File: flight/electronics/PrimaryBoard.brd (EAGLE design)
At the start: 90 x 90 mm, 14 parts

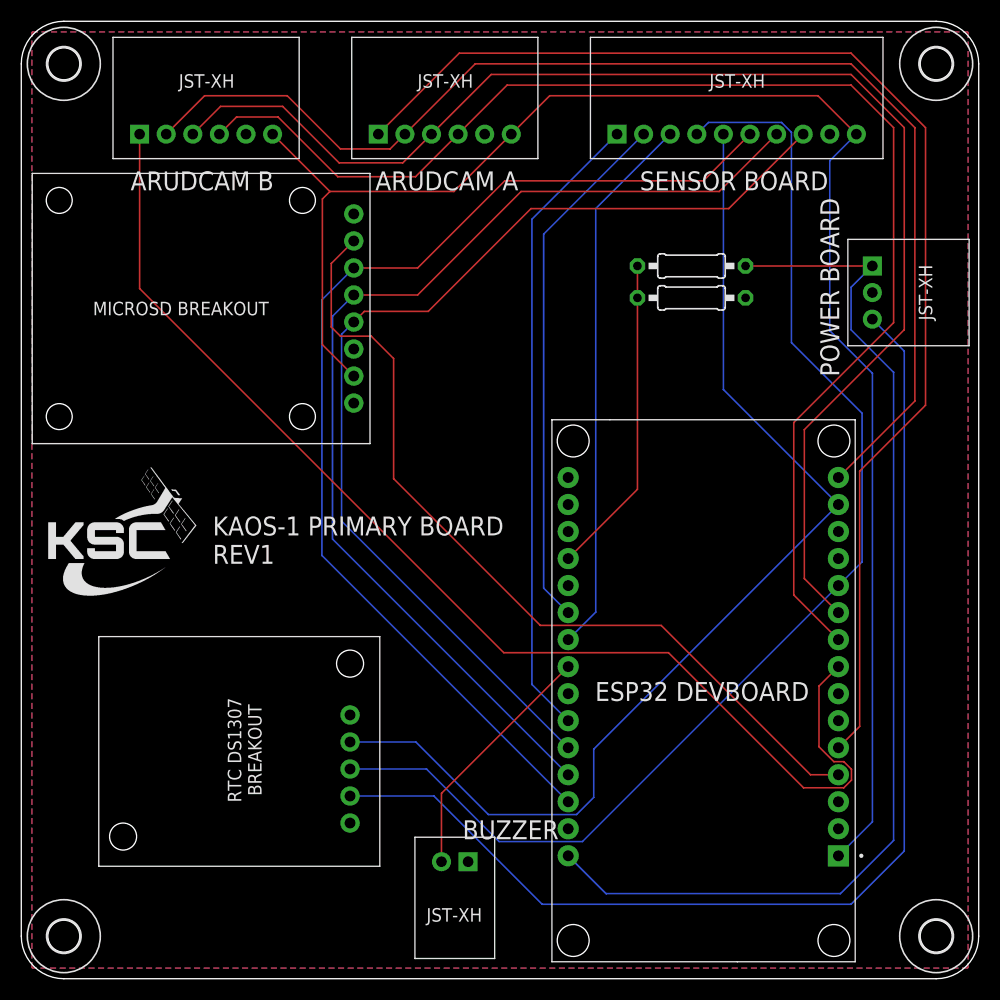
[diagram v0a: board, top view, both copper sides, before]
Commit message: primary board redesign
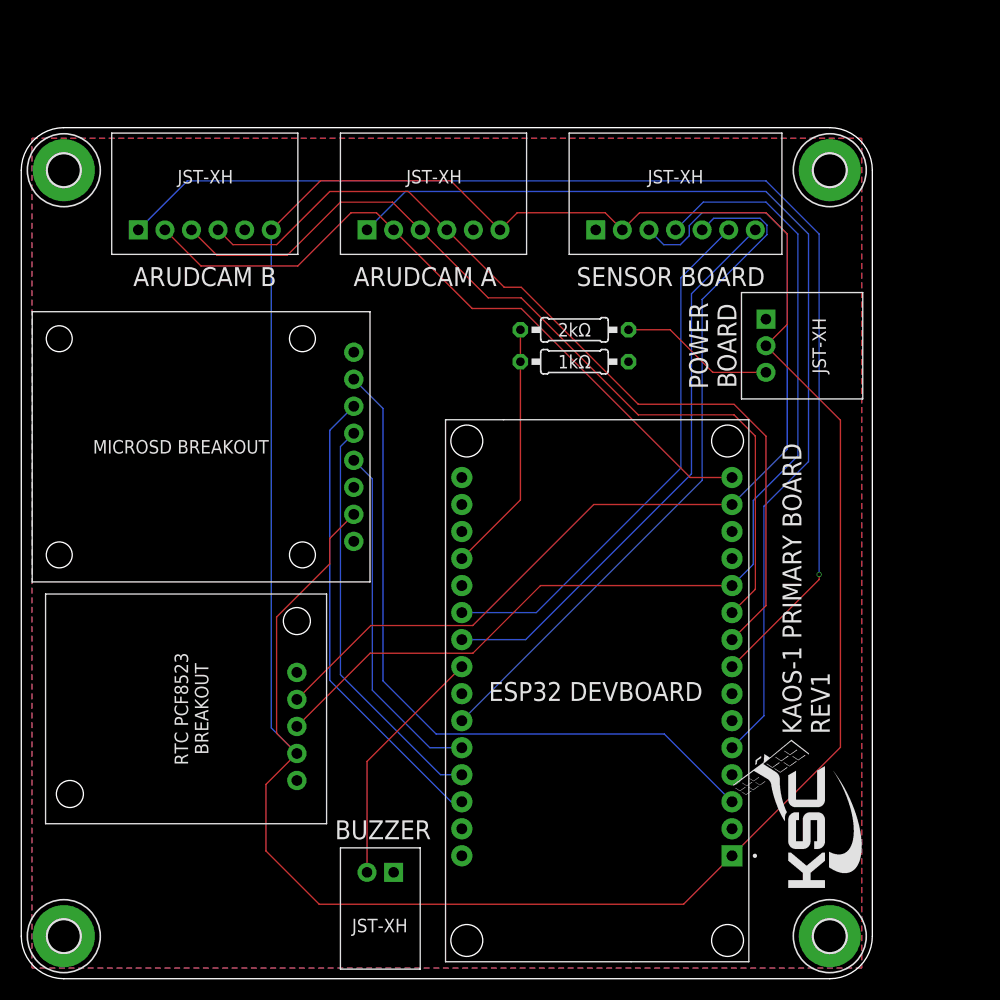
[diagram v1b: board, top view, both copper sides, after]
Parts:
- removed SENSOR_BOARD: JST-XH-10-PIN, Rembrandt Electronics - JST XH Connectors v1-0:JST-XH_S10B
- removed U$3, U$4, U$5, U$6: (no value), holes:3,0
- added H1, H2, H3, H4: MOUNT-PAD-ROUND3.0, holes:3,0-PAD
- added X1: JST-XH-07-PIN, Rembrandt Electronics - JST XH Connectors v1-0:JST-XH_S7B
- U$2: value DS1307BREAKOUT -> PCF8523BREAKOUT; device Breakouts:DS1307BREAKOUT -> Breakouts:PCF8523BREAKOUT
- moved U$1 13.0 mm to (15.0, 50.0)
- moved R1 12.5 mm to (52.0, 61.0)
- moved R2 12.5 mm to (52.0, 58.0)
- moved POWER_BOARD 11.2 mm to (70.0, 62.0)
- moved ESP32 10.0 mm to (54.1, 27.1)
- moved ARDUCAM-A 9.06 mm to (32.5, 70.4)
- moved ARDUCAM-B 9.00 mm to (11.0, 70.4)
- moved PIEZO 7.07 mm to (35.0, 10.0)
- moved U$2 6.40 mm to (16.0, 26.0)
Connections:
- removed net +5V: POWER_BOARD.PIN3, U$2.5V
- removed net MOSI_CLK: ESP32.26, SENSOR_BOARD.PIN8, U$1.CLK
- new net HSPI_CLK: ESP32.26, U$1.CLK
- net +3V3: now also POWER_BOARD.PIN2, U$2.VCC, X1.PIN2; no longer SENSOR_BOARD.PIN10
- net GND: now also H1.B3,0, H2.B3,0, H3.B3,0, H4.B3,0, POWER_BOARD.PIN1, X1.PIN1; no longer POWER_BOARD.PIN2, SENSOR_BOARD.PIN9
- net GPIO1: now also X1.PIN5; no longer SENSOR_BOARD.PIN1
- net GPIO2: now also X1.PIN6; no longer SENSOR_BOARD.PIN2
- net GPIO3: now also X1.PIN7; no longer SENSOR_BOARD.PIN3
- net HSPI_MISO: no longer SENSOR_BOARD.PIN7
- net HSPI_MOSI: no longer SENSOR_BOARD.PIN6
- net I2C_SCL: now also X1.PIN3; no longer SENSOR_BOARD.PIN5
- net I2C_SDA: now also X1.PIN4; no longer SENSOR_BOARD.PIN4
- net SD_CS: now also ESP32.3; no longer ESP32.4
- net VBAT: now also POWER_BOARD.PIN3; no longer ESP32.30, POWER_BOARD.PIN1
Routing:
- net +5V: track 109.6 -> 0.00 mm
- net +3V3: track 153.1 -> 256.2 mm
- net MOSI_CLK: track 98.9 -> 0.00 mm
- net VBAT: track 102.5 -> 14.6 mm
- net HSPI_MISO: track 101.1 -> 38.5 mm
- net HSPI_MOSI: track 103.5 -> 43.8 mm
- net VSPI_MOSI: track 115.6 -> 67.1 mm
- net VSPI_MISO: track 126.5 -> 82.7 mm
- net VSPI_CLK: track 125.3 -> 84.1 mm
- net HSPI_CLK: track 0.00 -> 33.0 mm
- net ARDUCAM-A_CS: track 119.2 -> 95.9 mm
- net I2C_SDA: track 114.7 -> 95.8 mm
- net SD_CS: track 80.7 -> 67.0 mm
- net I2C_SCL: track 102.7 -> 92.3 mm
- net BAT_MEASURE: track 30.2 -> 23.8 mm
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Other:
- board size 90 x 90 mm -> 80 x 80 mm

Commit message: final touches
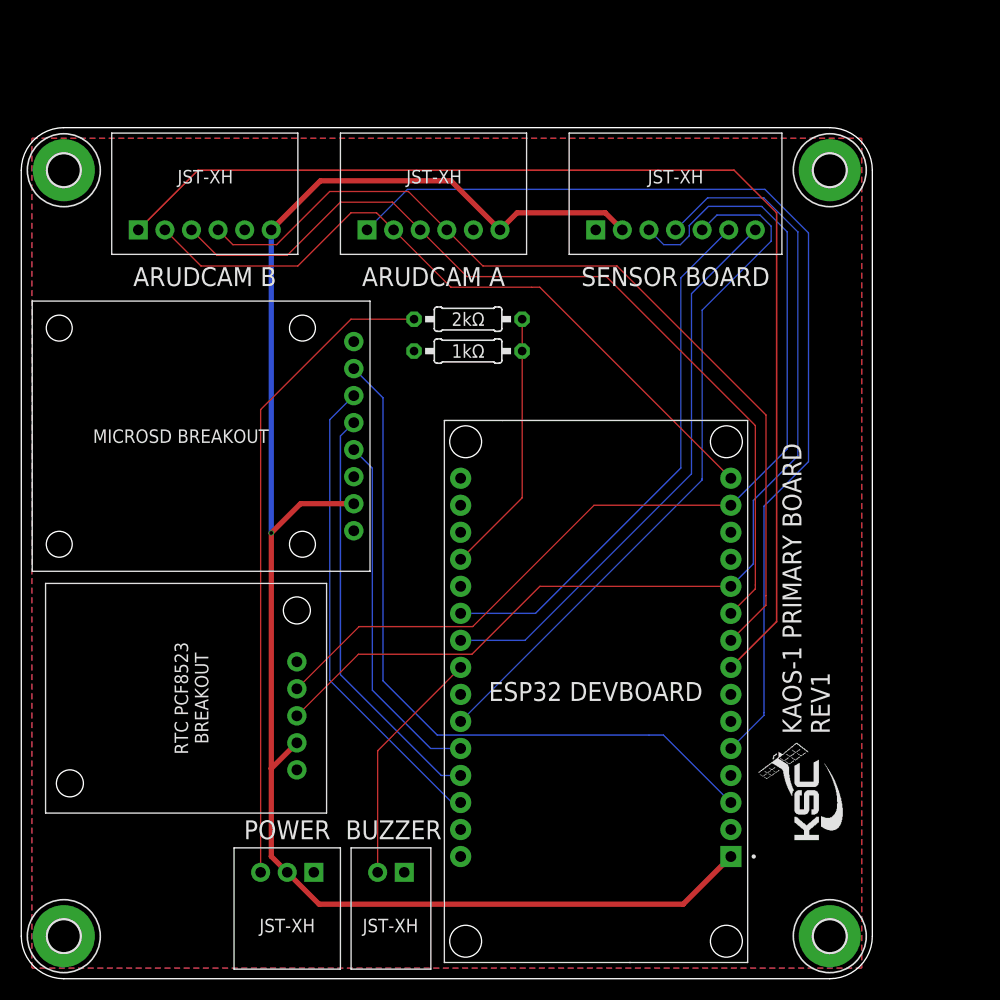
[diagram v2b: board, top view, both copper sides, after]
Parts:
- moved POWER_BOARD 67.2 mm to (27.5, 10.0), turned to 180 degrees
- moved R1 10.0 mm to (42.0, 62.0), turned to 0 degrees
- moved R2 10.0 mm to (42.0, 59.0), turned to 180 degrees
- moved PIEZO 1.00 mm to (36.0, 10.0)
- moved U$1 1.00 mm to (15.0, 51.0)
- moved U$2 1.00 mm to (16.0, 27.0)
- moved ESP32 0.13 mm to (54.0, 27.0)
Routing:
- net +3V3: track 256.2 -> 156.3 mm, vias 0 -> 1
- net VBAT: track 14.6 -> 61.4 mm
- net ARDUCAM-B_CS: track 112.0 -> 108.5 mm, vias 1 -> 0
- net VSPI_CLK: track 84.1 -> 85.4 mm
- net BAT_MEASURE: track 23.8 -> 25.0 mm
- net SD_CS: track 67.0 -> 67.9 mm
- net HSPI_MISO: track 38.5 -> 39.4 mm
- net HSPI_MOSI: track 43.8 -> 44.8 mm
- net HSPI_CLK: track 33.0 -> 33.9 mm
- net GPIO1: track 65.3 -> 66.1 mm
- net VSPI_MISO: track 82.7 -> 83.4 mm
- net PIEZO: track 23.0 -> 22.5 mm
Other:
- board text added: "POWER"
- board text removed: "POWER BOARD"

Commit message: final board tweaks
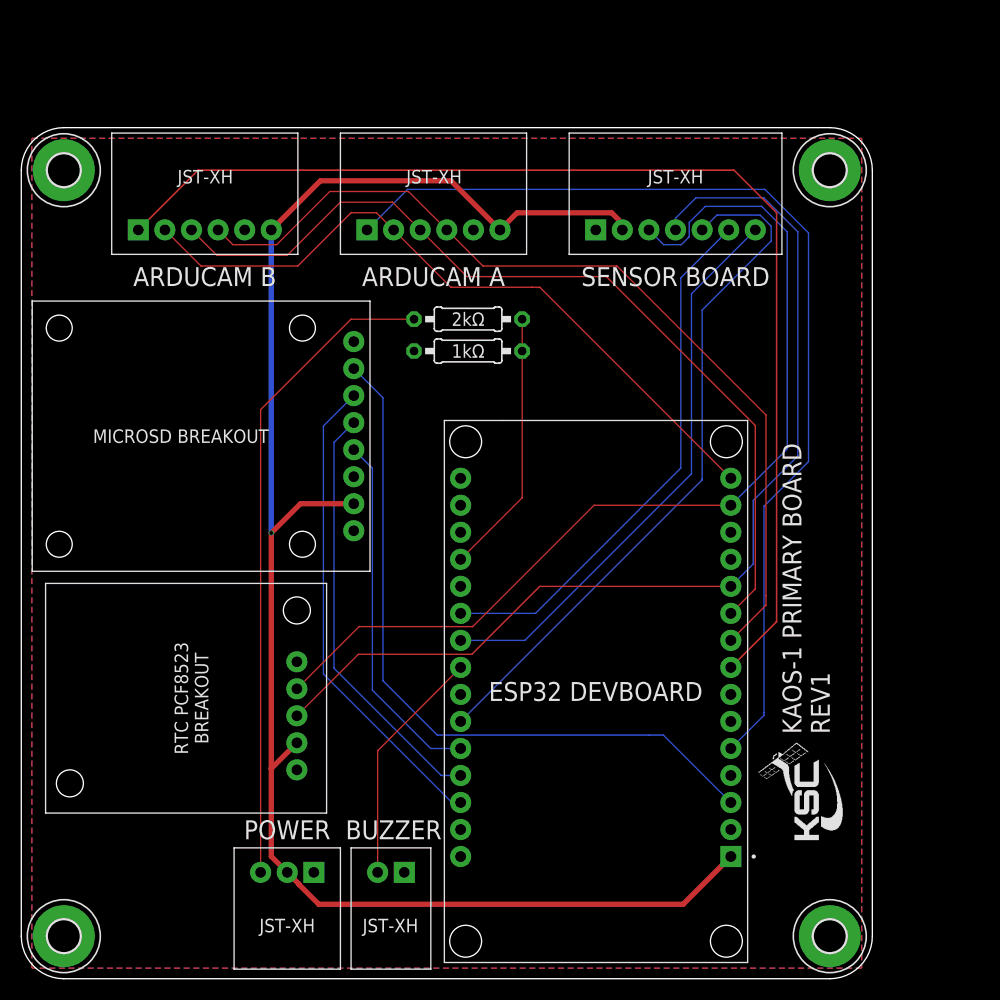
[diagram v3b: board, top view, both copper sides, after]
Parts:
- removed POWER_BOARD: JST-XH-03-PIN, Rembrandt Electronics - JST XH Connectors v1-0:JST-XH_S3B
- added X2: JST-XH-03-PIN, JST-XH Connectors:JST-XH_S3B
- ARDUCAM-A, ARDUCAM-B: device Rembrandt Electronics - JST XH Connectors v1-0:JST-XH_S6B -> JST-XH Connectors:JST-XH_S6B
- PIEZO: device Rembrandt Electronics - JST XH Connectors v1-0:JST-XH_S2B -> JST-XH Connectors:JST-XH_S2B
- X1: device Rembrandt Electronics - JST XH Connectors v1-0:JST-XH_S7B -> JST-XH Connectors:JST-XH_S7B
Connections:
- net +3V3: now also X2.PIN2; no longer POWER_BOARD.PIN2
- net GND: now also X2.PIN1; no longer POWER_BOARD.PIN1
- net VBAT: now also X2.PIN3; no longer POWER_BOARD.PIN3
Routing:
- net I2C_SDA: track 95.8 -> 96.5 mm
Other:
- board text added: "ARDUCAM A"
- board text added: "ARDUCAM B"
- board text removed: "ARUDCAM A"
- board text removed: "ARUDCAM B"

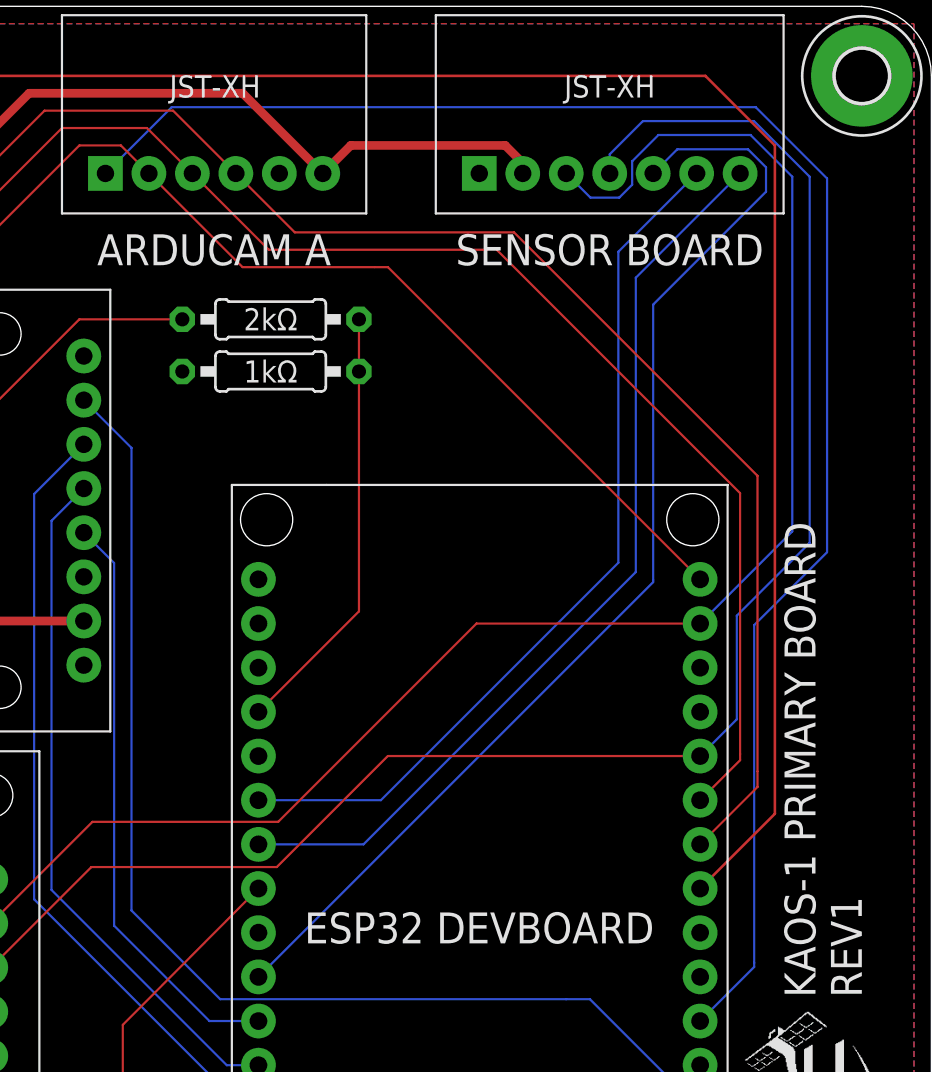
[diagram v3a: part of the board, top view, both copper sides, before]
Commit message: rev1 changes
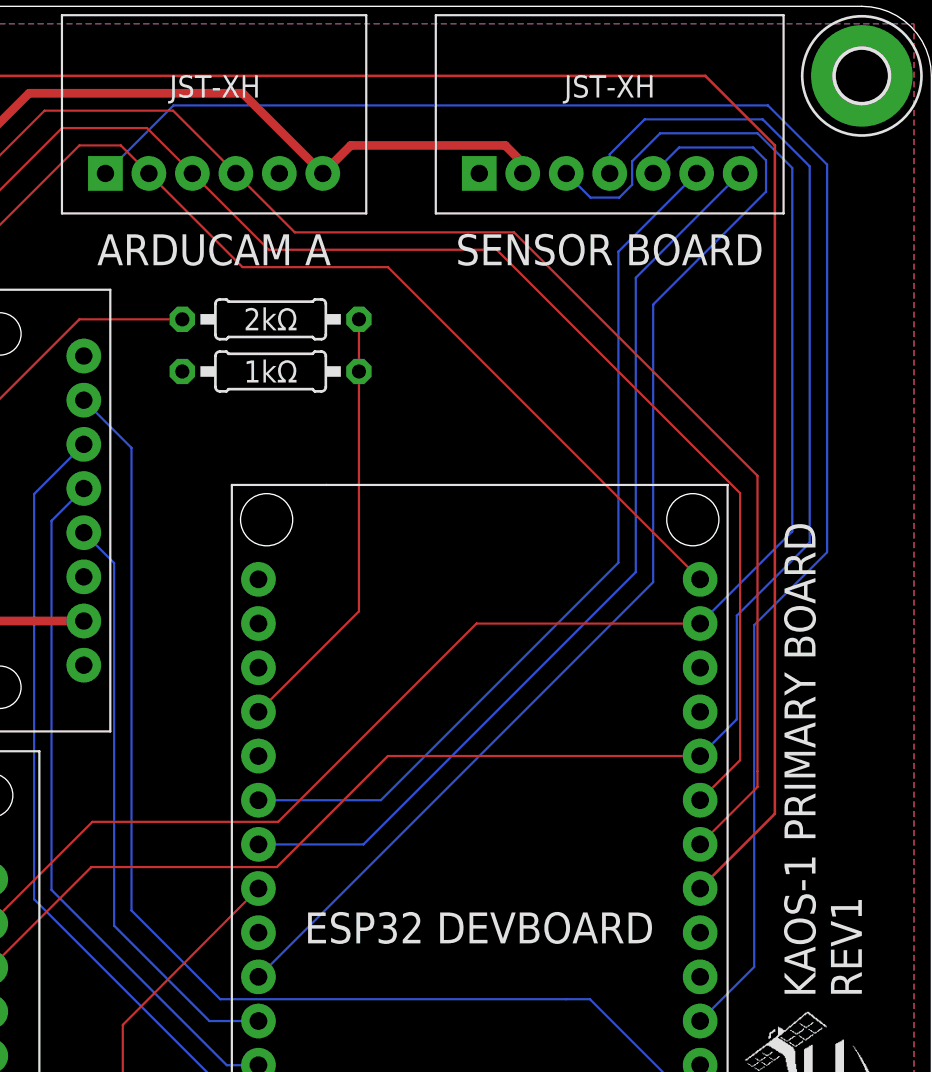
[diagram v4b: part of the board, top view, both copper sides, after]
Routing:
- net ARDUCAM-A_CS: track 96.3 -> 96.8 mm
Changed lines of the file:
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@@
 <drawing>
 <settings>
-<setting alwaysvectorfont="no"/>
+<setting alwaysvectorfont="yes"/>
 <setting verticaltext="up"/>
 </settings>
@@
 <wire x1="59" y1="70.39" x2="60.39" y2="69" width="0.127" layer="16"/>
 <wire x1="62.7905" y1="69.7383" x2="62.7905" y2="71.0905" width="0.127" layer="16"/>
-<wire x1="62.7905" y1="71.0905" x2="64.3" y2="72.6" width="0.127" layer="16"/>
-<wire x1="64.3" y1="72.6" x2="69.6" y2="72.6" width="0.127" layer="16"/>
-<wire x1="69.6" y1="72.6" x2="72" y2="70.2" width="0.127" layer="16"/>
-<wire x1="72" y1="70.2" x2="72" y2="49.805" width="0.127" layer="16"/>
+<wire x1="62.7905" y1="71.0905" x2="64.4" y2="72.7" width="0.127" layer="16"/>
+<wire x1="64.4" y1="72.7" x2="70" y2="72.7" width="0.127" layer="16"/>
+<wire x1="70" y1="72.7" x2="72" y2="70.7" width="0.127" layer="16"/>
+<wire x1="72" y1="70.7" x2="72" y2="49.805" width="0.127" layer="16"/>
 <wire x1="60.39" y1="69" x2="62.0522" y2="69" width="0.127" layer="16"/>
 <wire x1="62.0522" y1="69" x2="62.7905" y2="69.7383" width="0.127" layer="16"/>
@@
 <wire x1="48.74" y1="36.885" x2="42.355" y2="30.5" width="0.127" layer="1"/>
 <wire x1="31.692" y1="30.5" x2="42.355" y2="30.5" width="0.127" layer="1"/>
-<wire x1="63.41" y1="73.4" x2="61.5" y2="71.49" width="0.127" layer="16"/>
+<wire x1="63.51" y1="73.5" x2="61.5" y2="71.49" width="0.127" layer="16"/>
 <wire x1="61.5" y1="70.39" x2="61.5" y2="71.49" width="0.127" layer="16"/>
-<wire x1="69.8" y1="73.4" x2="73" y2="70.2" width="0.127" layer="16"/>
-<wire x1="73" y1="70.2" x2="73" y2="49.145" width="0.127" layer="16"/>
+<wire x1="70.3" y1="73.5" x2="73" y2="70.8" width="0.127" layer="16"/>
+<wire x1="73" y1="70.8" x2="73" y2="49.145" width="0.127" layer="16"/>
 <wire x1="68.81" y1="44.955" x2="73" y2="49.145" width="0.127" layer="16"/>
-<wire x1="63.41" y1="73.4" x2="69.8" y2="73.4" width="0.127" layer="16"/>
+<wire x1="63.51" y1="73.5" x2="70.3" y2="73.5" width="0.127" layer="16"/>
 <contactref element="U$2" pad="SDA"/>
 <contactref element="X1" pad="PIN4"/>
@@
 </signal>
 <signal name="GPIO1">
-<wire x1="69.4517" y1="71.7805" x2="70.4905" y2="70.7417" width="0.127" layer="16"/>
-<wire x1="70.4905" y1="70.7417" x2="70.4905" y2="69.3383" width="0.127" layer="16"/>
-<wire x1="64" y1="62.8478" x2="64" y2="47" width="0.127" layer="16"/>
+<wire x1="69.7517" y1="71.8805" x2="70.4905" y2="71.1417" width="0.127" layer="16"/>
+<wire x1="70.4905" y1="71.1417" x2="70.4905" y2="69.3383" width="0.127" layer="16"/>
+<wire x1="64" y1="62.8478" x2="64" y2="46.885" width="0.127" layer="16"/>
 <wire x1="70.4905" y1="69.3383" x2="64" y2="62.8478" width="0.127" layer="16"/>
-<wire x1="64" y1="70.39" x2="65.3905" y2="71.7805" width="0.127" layer="16"/>
-<wire x1="65.3905" y1="71.7805" x2="69.4517" y2="71.7805" width="0.127" layer="16"/>
+<wire x1="64" y1="70.39" x2="65.4905" y2="71.8805" width="0.127" layer="16"/>
+<wire x1="65.4905" y1="71.8805" x2="69.7517" y2="71.8805" width="0.127" layer="16"/>
 <contactref element="X1" pad="PIN5"/>
 <contactref element="ESP32" pad="25"/>
 <wire x1="41.3" y1="24.185" x2="64" y2="46.885" width="0.127" layer="16"/>
-<wire x1="64" y1="46.885" x2="64" y2="47" width="0.127" layer="16"/>
 </signal>
 <signal name="VSPI_CLK">
@@
 </signal>
 <signal name="ARDUCAM-A_CS">
-<wire x1="32.5" y1="70.39" x2="36.31" y2="74.2" width="0.127" layer="16"/>
-<wire x1="69.9" y1="74.2" x2="74" y2="70.1" width="0.127" layer="16"/>
-<wire x1="74" y1="70.1" x2="74" y2="48.605" width="0.127" layer="16"/>
+<wire x1="32.5" y1="70.39" x2="36.41" y2="74.3" width="0.127" layer="16"/>
+<wire x1="70.6" y1="74.3" x2="74" y2="70.9" width="0.127" layer="16"/>
+<wire x1="74" y1="70.9" x2="74" y2="48.605" width="0.127" layer="16"/>
 <wire x1="74" y1="48.605" x2="69.81" y2="44.415" width="0.127" layer="16"/>
-<wire x1="69.81" y1="44.415" x2="69.81" y2="25" width="0.127" layer="16"/>
-<wire x1="36.31" y1="74.2" x2="69.9" y2="74.2" width="0.127" layer="16"/>
+<wire x1="69.81" y1="44.415" x2="69.81" y2="24.755" width="0.127" layer="16"/>
+<wire x1="36.41" y1="74.3" x2="70.6" y2="74.3" width="0.127" layer="16"/>
 <contactref element="ARDUCAM-A" pad="PIN1"/>
 <contactref element="ESP32" pad="5"/>
 <wire x1="66.7" y1="21.645" x2="69.81" y2="24.755" width="0.127" layer="16"/>
-<wire x1="69.81" y1="24.755" x2="69.81" y2="25" width="0.127" layer="16"/>
 </signal>
 <signal name="SD_CS">
